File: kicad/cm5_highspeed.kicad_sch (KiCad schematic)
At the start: 10 parts, among them J16 Conn_01x22_Female, J5 Conn_01x22_Female, U1 467651001, U4 RT9742SNGV

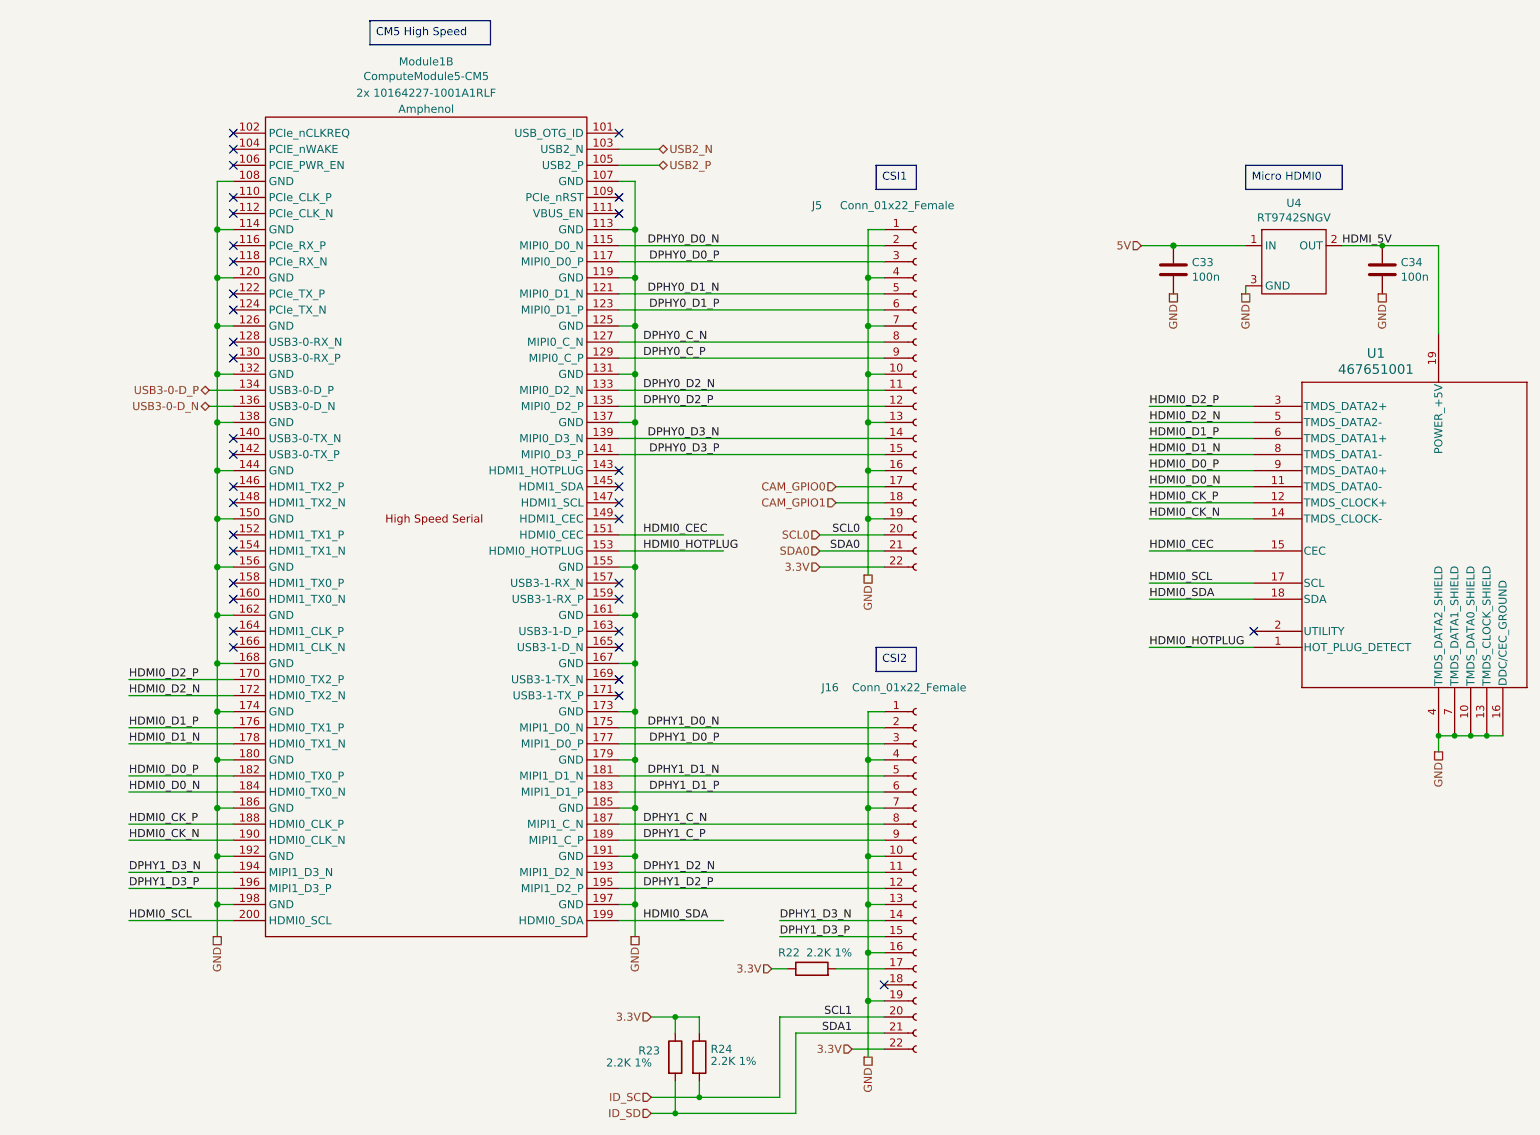
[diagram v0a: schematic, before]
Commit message: finish first pcb revision
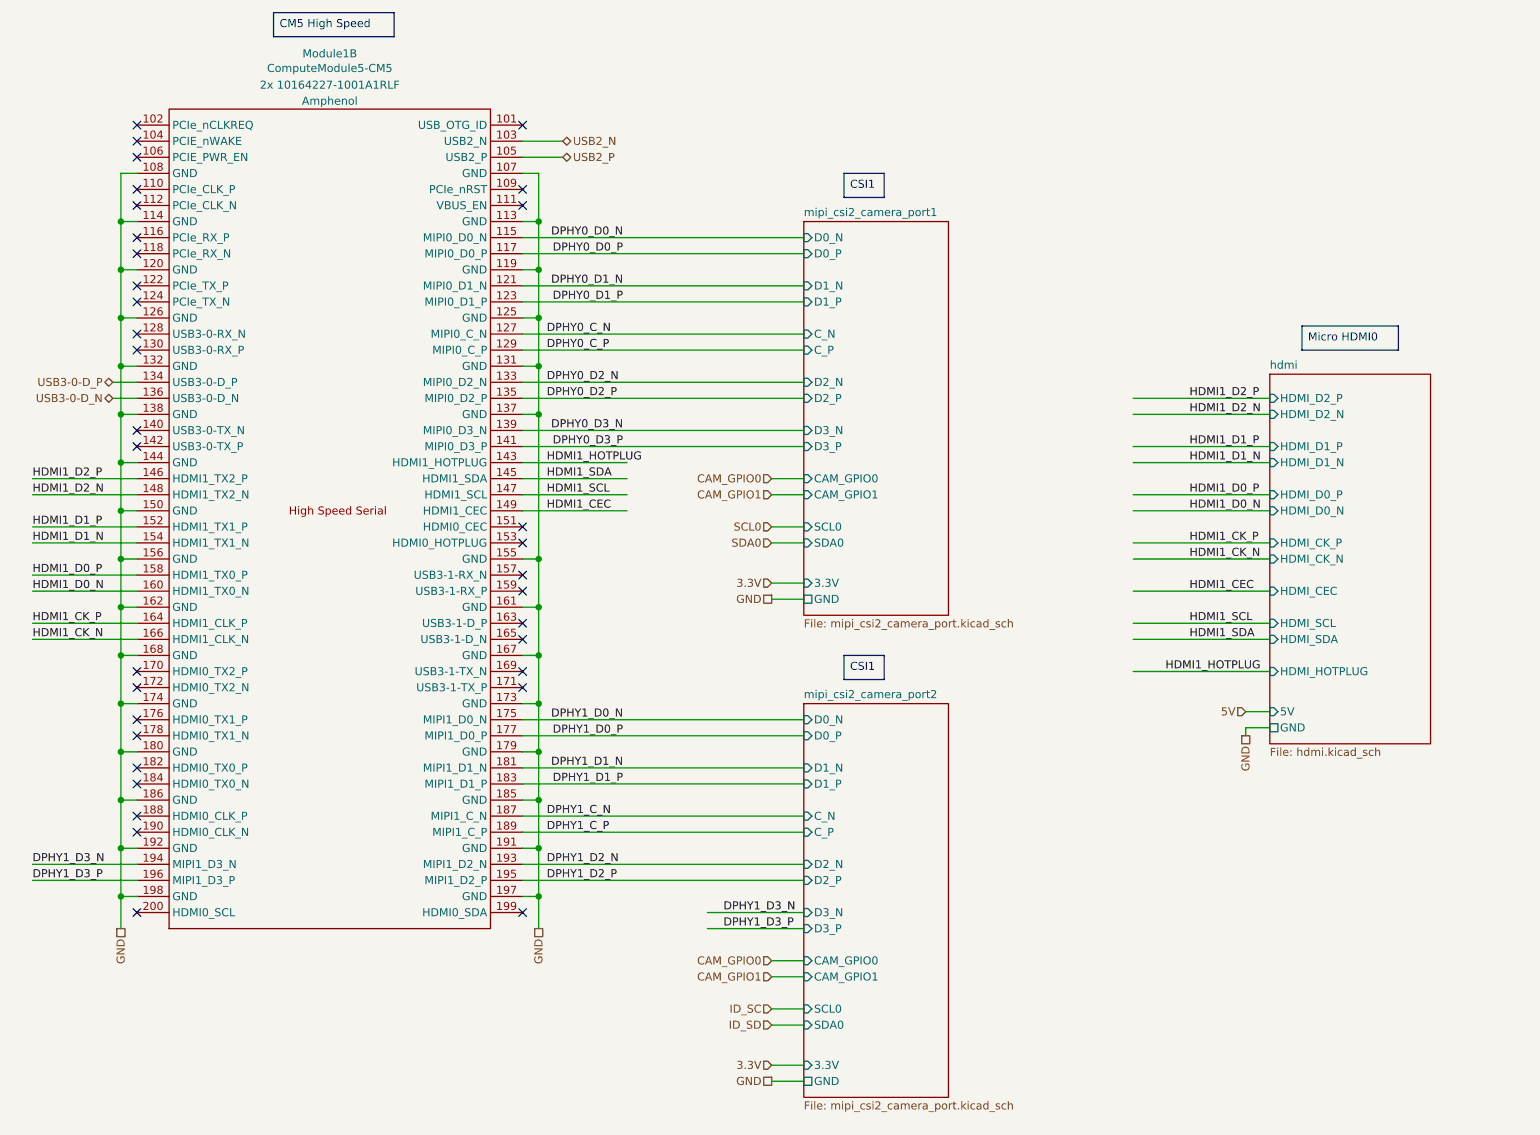
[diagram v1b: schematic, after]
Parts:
- removed C33, C34: 100n, Capacitor_SMD:C_0402_1005Metric, symbol Device:C
- removed J16, J5: Conn_01x22_Female, CM5IO:Hirose_FH12-22S-0.5SH_1x22-1MP_P0.50mm_Horizontal, symbol Connector:Conn_01x22_Socket
- removed R22, R23, R24: 2.2K 1%, Resistor_SMD:R_0402_1005Metric, symbol Device:R
- removed U1: 467651001, symbol 467651001:467651001
- removed U4: RT9742SNGV, Package_TO_SOT_SMD:TSOT-23_HandSoldering, symbol CM5IO:RT9742SNGV
- Module1: footprint CM5IO:Raspberry-Pi-5-Compute-Module -> CM5:Raspberry-Pi-5-Compute-Module
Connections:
- net HDMI1_HOTPLUG: now reaches Module1.143 (HDMI1_HOTPLUG)
- net HDMI1_SDA: now reaches Module1.145 (HDMI1_SDA)
- net HDMI1_D2_P: now reaches Module1.146 (HDMI1_TX2_P)
- net HDMI1_SCL: now reaches Module1.147 (HDMI1_SCL)
- net HDMI1_D2_N: now reaches Module1.148 (HDMI1_TX2_N)
- net HDMI1_CEC: now reaches Module1.149 (HDMI1_CEC)
- net HDMI1_D1_P: now reaches Module1.152 (HDMI1_TX1_P)
- net HDMI1_D1_N: now reaches Module1.154 (HDMI1_TX1_N)
- net HDMI1_D0_P: now reaches Module1.158 (HDMI1_TX0_P)
- net HDMI1_D0_N: now reaches Module1.160 (HDMI1_TX0_N)
- net HDMI1_CK_P: now reaches Module1.164 (HDMI1_CLK_P)
- net HDMI1_CK_N: now reaches Module1.166 (HDMI1_CLK_N)
- net HDMI0_CEC: no longer names the net of Module1.151 (HDMI0_CEC)
- net HDMI0_CK_N: no longer names the net of Module1.190 (HDMI0_CLK_N)
- net HDMI0_CK_P: no longer names the net of Module1.188 (HDMI0_CLK_P)
- net HDMI0_D0_N: no longer names the net of Module1.184 (HDMI0_TX0_N)
- net HDMI0_D0_P: no longer names the net of Module1.182 (HDMI0_TX0_P)
- net HDMI0_D1_N: no longer names the net of Module1.178 (HDMI0_TX1_N)
- net HDMI0_D1_P: no longer names the net of Module1.176 (HDMI0_TX1_P)
- net HDMI0_D2_N: no longer names the net of Module1.172 (HDMI0_TX2_N)
- net HDMI0_D2_P: no longer names the net of Module1.170 (HDMI0_TX2_P)
- net HDMI0_HOTPLUG: no longer names the net of Module1.153 (HDMI0_HOTPLUG)
- net HDMI0_SCL: no longer names the net of Module1.200 (HDMI0_SCL)
- net HDMI0_SDA: no longer names the net of Module1.199 (HDMI0_SDA)
- no-connect marks 36 -> 34
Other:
- added sheet hdmi (hdmi.kicad_sch)
- added sheet mipi_csi2_camera_port1 (mipi_csi2_camera_port.kicad_sch)
- added sheet mipi_csi2_camera_port2 (mipi_csi2_camera_port.kicad_sch)
- moved on the sheet: Module1B
